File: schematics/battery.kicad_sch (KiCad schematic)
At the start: 6 parts

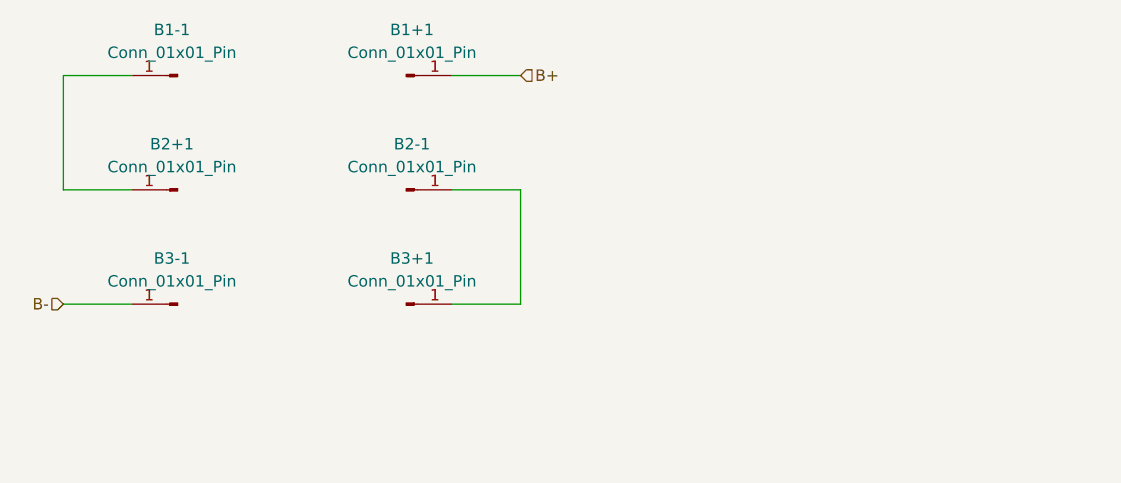
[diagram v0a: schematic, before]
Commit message: stand 14:40 24.11.2025
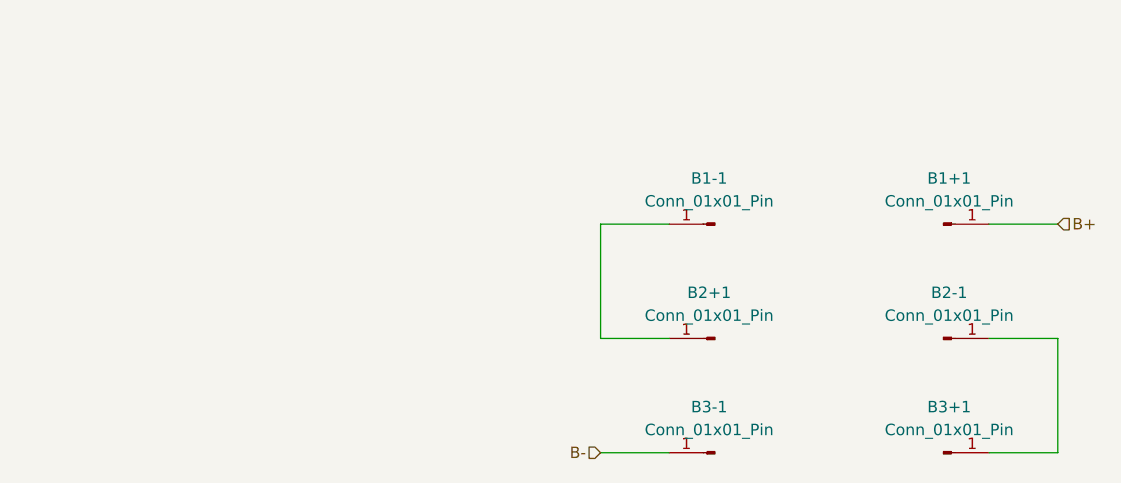
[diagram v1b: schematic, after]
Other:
- company: (none) -> Rücklicht 4
- title: (none) -> Rücklicht
- moved on the sheet: B1+1, B1-1, B2+1, B2-1, B3+1, B3-1
